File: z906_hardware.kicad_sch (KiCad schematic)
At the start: 16 parts, among them J1 USB_C_Receptacle_USB2.0_14P, J3 DE_15 Amplifier, J4 DE15 Console, U1 ESP32-S3-WROOM-1, U2 ME6211C33M5, U3 PCM5102A

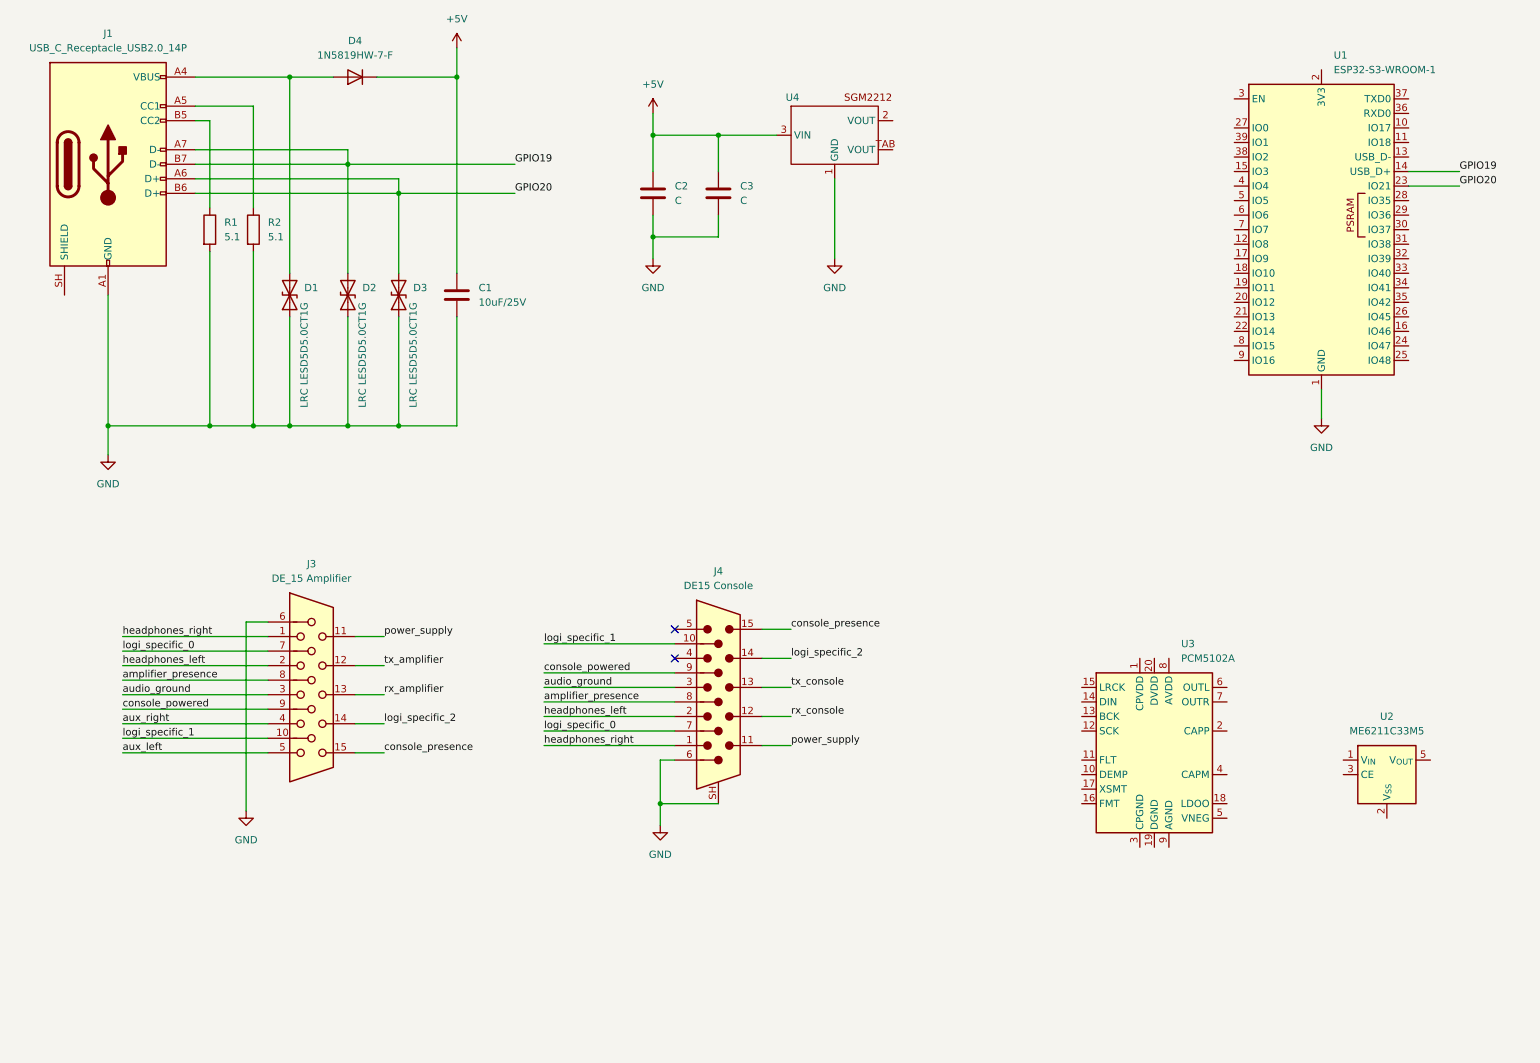
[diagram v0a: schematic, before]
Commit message: esp32-s3
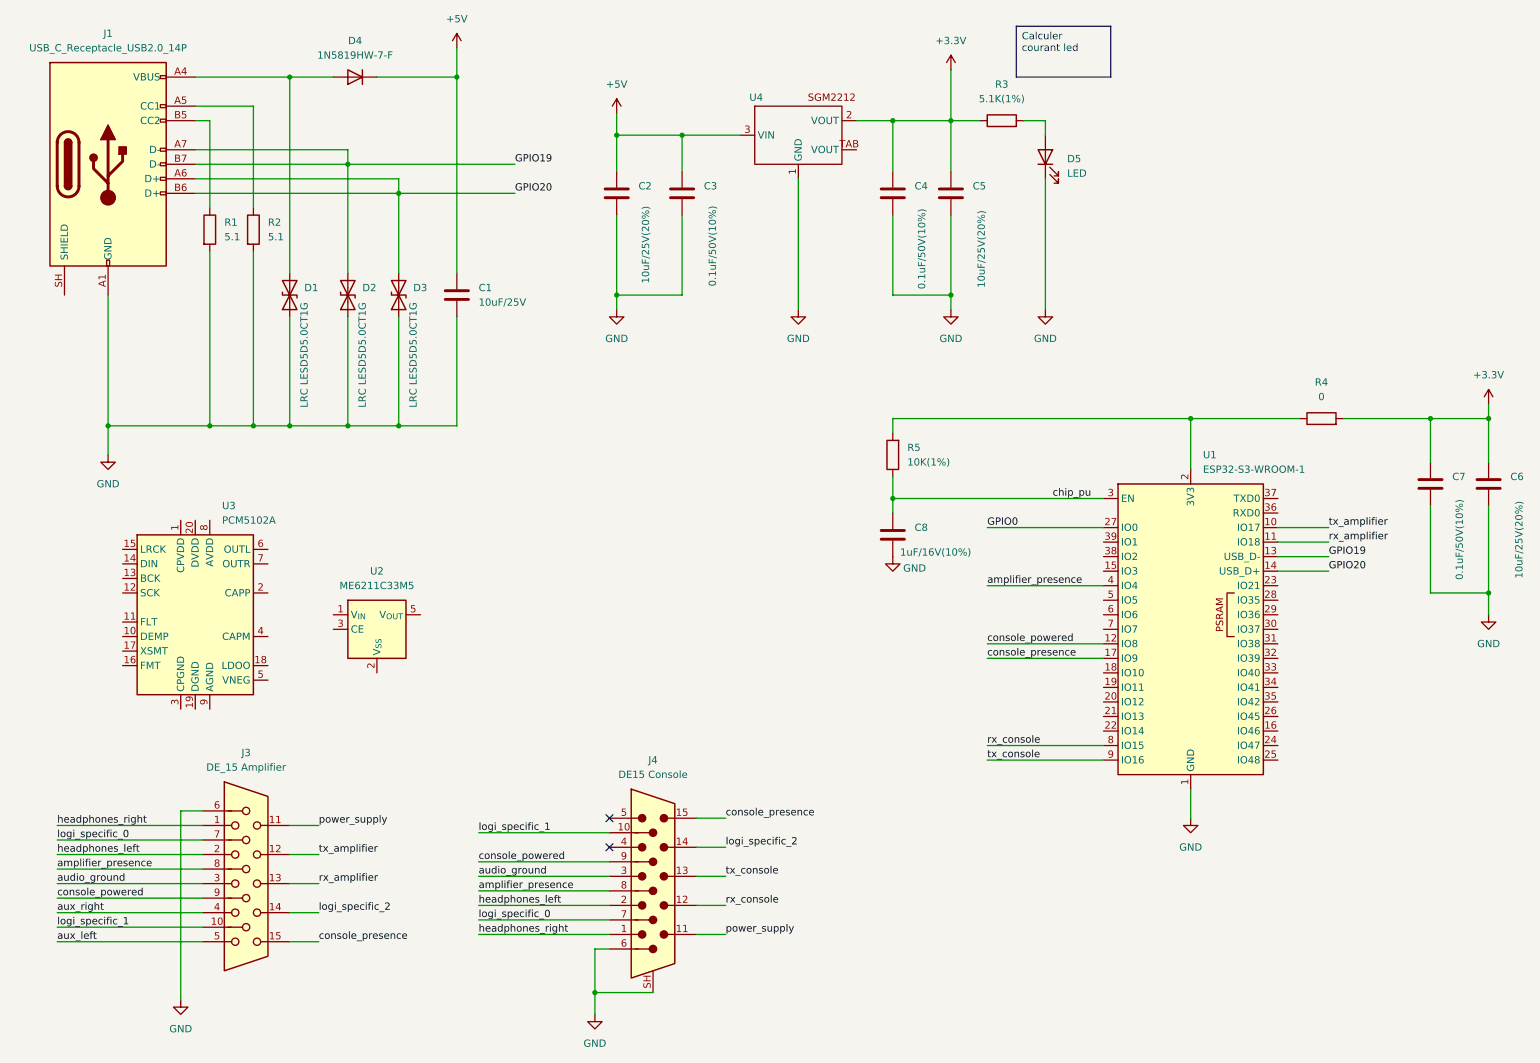
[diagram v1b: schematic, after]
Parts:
- added C4, C7: 0.1uF/50V(10%), symbol Device:C
- added C5, C6: 10uF/25V(20%), symbol Device:C
- added C8: 1uF/16V(10%), symbol Device:C
- added D5: LED, symbol Device:LED
- added R3: 5.1K(1%), symbol Device:R
- added R4: 0, symbol Device:R
- added R5: 10K(1%), symbol Device:R
- C2: value C -> 10uF/25V(20%)
- C3: value C -> 0.1uF/50V(10%)
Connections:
- net GND: now also C4.2, C5.2, C6.2, C7.2, C8.2, D5.1 (K)
- net GPIO19: now also U1.13 (USB_D-); no longer U1.14 (USB_D+)
- net GPIO20: now also U1.14 (USB_D+); no longer U1.23 (IO21)
- net amplifier_presence: now also U1.4 (IO4)
- net console_powered: now also U1.12 (IO8)
- net console_presence: now also U1.17 (IO9)
- net rx_amplifier: now also U1.11 (IO18)
- net rx_console: now also U1.8 (IO15)
- net tx_amplifier: now also U1.10 (IO17)
- net tx_console: now also U1.9 (IO16)
- net +3.3V: now reaches U4.2 (VOUT)
- net +3.3V: now also C4.1, C5.1, C6.1, C7.1, R3.1, R4.2
- net at U1.2 (3V3): now also R4.1, R5.2
- net GPIO0: now reaches U1.27 (IO0)
- net chip_pu: now reaches U1.3 (EN)
- net chip_pu: now also C8.1, R5.1
- new net: D5.2 (A), R3.2
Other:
- moved on the sheet: C2, C3, J3, J4, U1, U2, U3, U4
